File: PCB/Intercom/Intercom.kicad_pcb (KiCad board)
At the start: 2 copper layers, 70 x 70 mm, 73 parts, among them J1 Reset, J2 JST-PH-SM4-TB, J4 TC2030-USB-NL-DS, J5 USB-C-Socket-H, P1 Square, P2 Square, SW1 SW_SPST, U1 MD8942, U2 ESP32-S3-MINI-1, U4 ICS43434, U6 MAX98357A

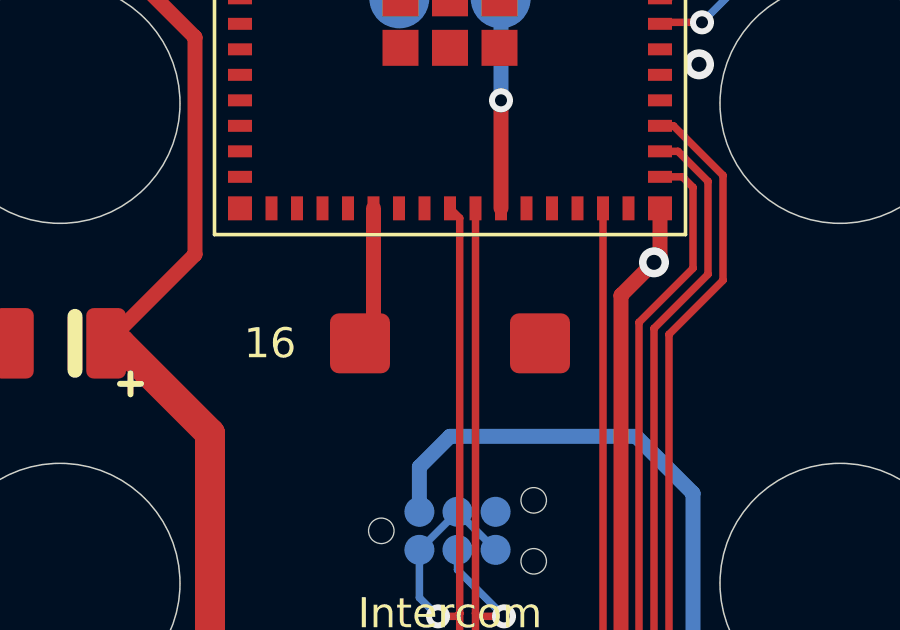
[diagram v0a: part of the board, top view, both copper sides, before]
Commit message: Render
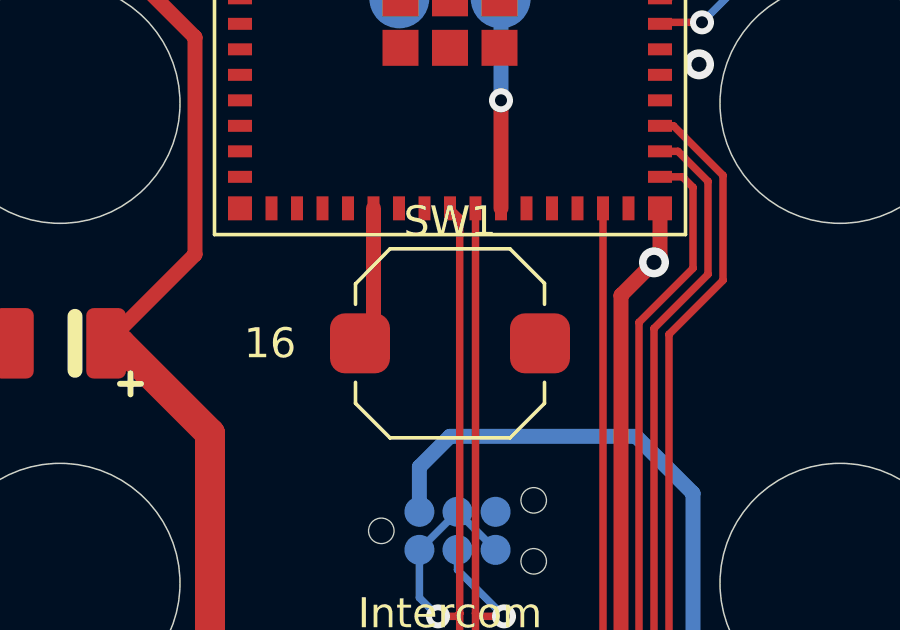
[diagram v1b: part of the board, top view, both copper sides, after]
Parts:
- SW1: footprint RevK:SPEH130103 -> Button_Switch_SMD:SW_Push_1TS009xxxx-xxxx-xxxx_6x6x5mm
